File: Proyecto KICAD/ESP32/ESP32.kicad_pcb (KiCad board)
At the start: 2 copper layers, 34 parts, among them J1 Conn_01x17, J2 Conn_01x17, J3 USB_B_Micro, Q1 BC847, Q2 BC847, SW1 SW_Push, SW2 SW_Push, U1 esp32-devkitM-1, U2 CP2102N-Axx-xQFN28, U3 SGM2212-3.3XKC3G/TR

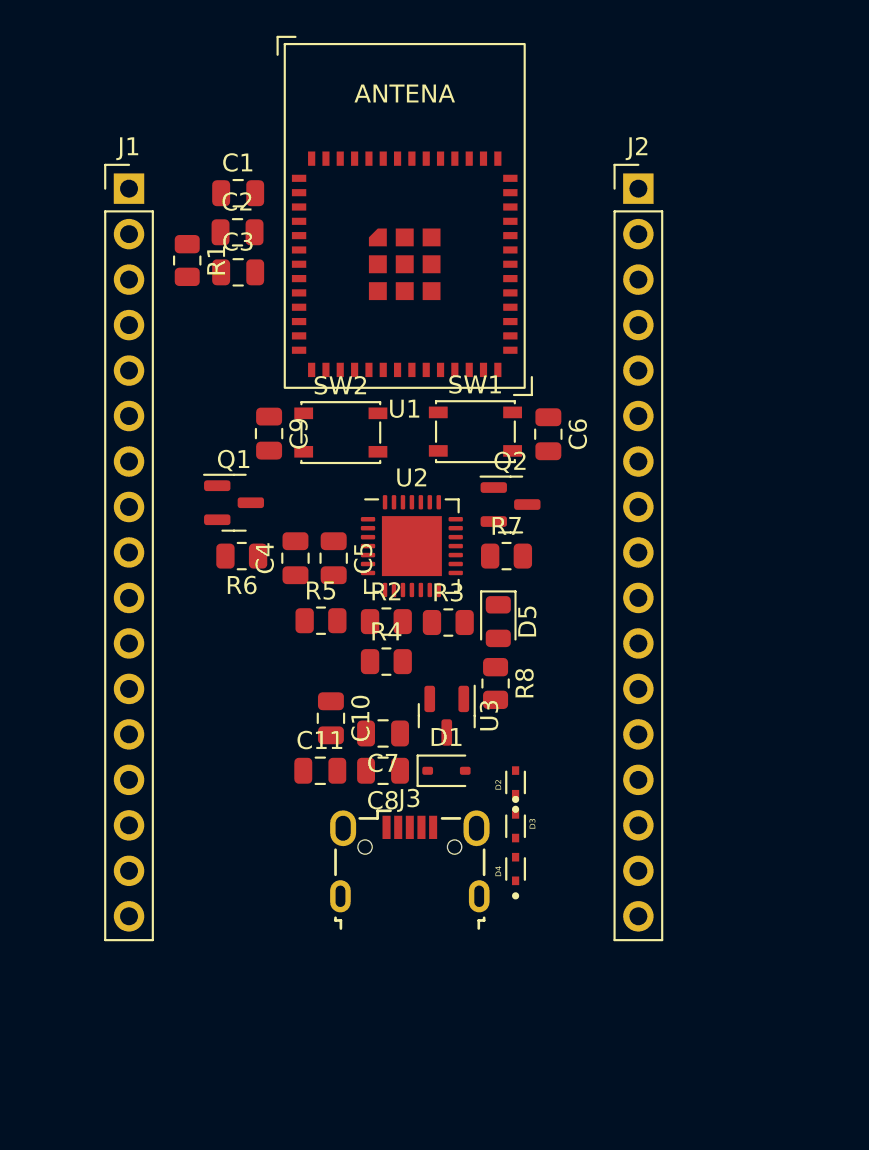
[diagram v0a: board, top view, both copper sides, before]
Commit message: c
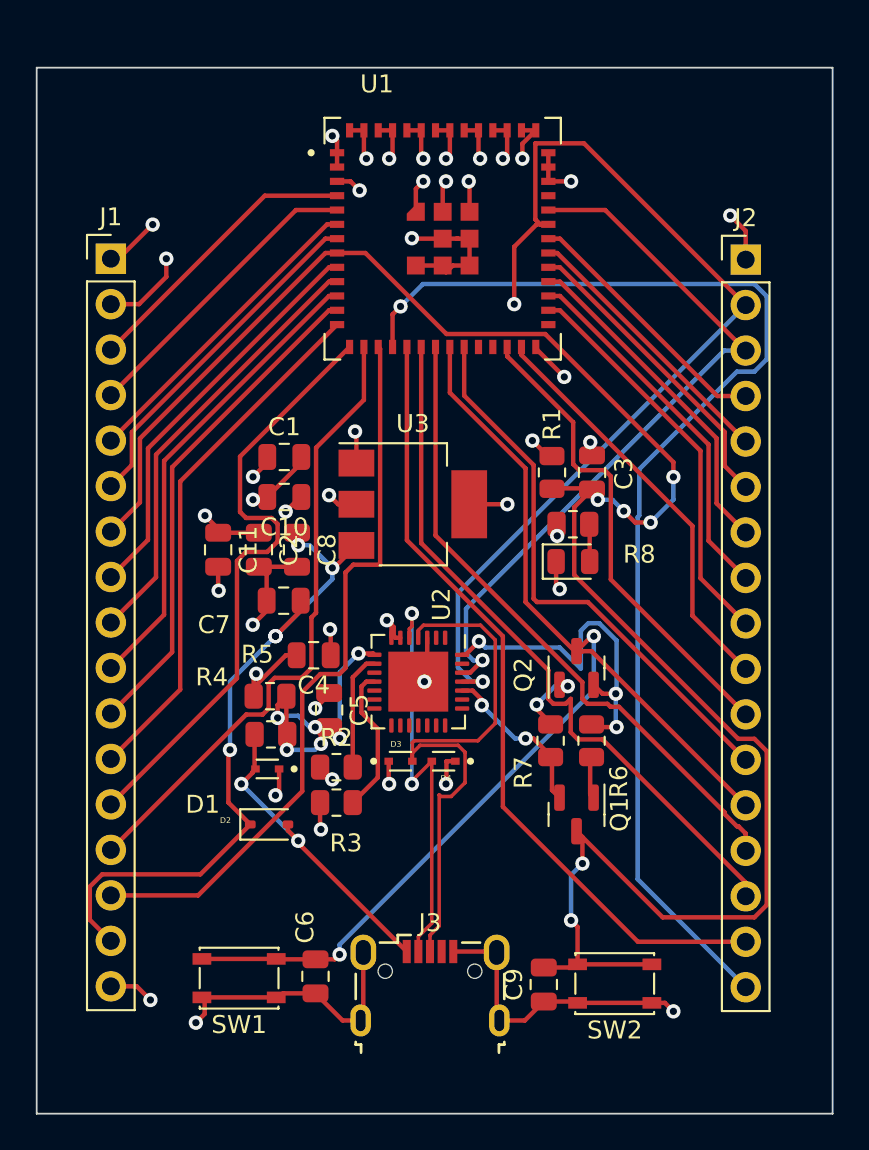
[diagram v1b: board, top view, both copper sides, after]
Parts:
- U1: footprint nuevas huella:esp32-devkitM-1 -> ESP32-MINI-1U-N4 (3):MODULE_ESP32-MINI-1U-N4
- U3: footprint Package_TO_SOT_SMD:SOT-23 -> Package_TO_SOT_SMD:SOT-223-3_TabPin2
- moved C9 34.4 mm to (182.6, 131.2), turned to 90 degrees
- moved SW2 34.4 mm to (186.6, 131.2), turned to 180 degrees
- moved SW1 33.3 mm to (165.6, 130.9), turned to 180 degrees
- moved C6 33.0 mm to (169.9, 130.8), turned to 90 degrees
- moved Q1 25.9 mm to (184.5, 121.7), turned to -90 degrees
- moved R1 23.6 mm to (183.1, 102.6)
- moved C3 22.7 mm to (185.3, 102.6), turned to 90 degrees
- moved R6 22.1 mm to (185.3, 117.6), turned to -90 degrees
- moved C2 17.8 mm to (166.7, 106.9), turned to -90 degrees
- moved C1 15.0 mm to (168.1, 101.8)
- moved D2 13.9 mm to (167.2, 119.2), turned to 180 degrees
- moved C11 13.6 mm to (164.4, 106.9), turned to -90 degrees
- moved C8 13.2 mm to (168.8, 106.9), turned to -90 degrees
- moved C10 12.6 mm to (168.1, 104.0), turned to 180 degrees
- moved U3 12.0 mm to (175.3, 104.4), turned to 0 degrees
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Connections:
- C10 pad 1: +3V3 -> +3.3V
- C11 pad 1: +3V3 -> +3.3V
- R8 pad 2: +3V3 -> +3.3V
- U1 pad 3: unconnected-(U1-3V3-Pad3) -> +3.3V
- U3 pad 2: +3V3 -> +3.3V
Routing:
- net ESP_RST: track 0.00 -> 111.2 mm, vias 0 -> 6
- net GND: track 0.00 -> 108.4 mm, vias 0 -> 32
- net GPIO12: track 0.00 -> 68.3 mm, vias 0 -> 1
- net GPIO0: track 0.00 -> 66.0 mm, vias 0 -> 2
- net U0RXD: track 0.00 -> 56.0 mm, vias 0 -> 2
- net GPIO13: track 0.00 -> 44.6 mm
- net GPIO14: track 0.00 -> 41.3 mm
- net U0TXD: track 0.00 -> 40.9 mm, vias 0 -> 1
- net GPIO15: track 0.00 -> 40.0 mm
- net +5V: track 0.00 -> 38.7 mm, vias 0 -> 5
- net GPIO2: track 0.00 -> 36.3 mm
- net GPIO27: track 0.00 -> 35.4 mm
- net GPIO26: track 0.00 -> 34.3 mm
- net USB_DP: track 0.00 -> 32.1 mm
- net GPIO4: track 0.00 -> 31.2 mm
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- added copper zone on In2.Cu, net +3.3V
- added copper zone on In1.Cu, net GND
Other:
- board outline added: 44.4 x 58.4 mm
- copper layers 2 -> 4
